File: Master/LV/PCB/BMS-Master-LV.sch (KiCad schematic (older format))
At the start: 24 parts, among them J10 Charge, J11 CAN, J12 USB, J13 Master, J18 OLED, J4 Power, J5 12V, J6 Power Button, J7 Cooling, J8 Discharge, K1 HE3621A1200, Q1 BSS138

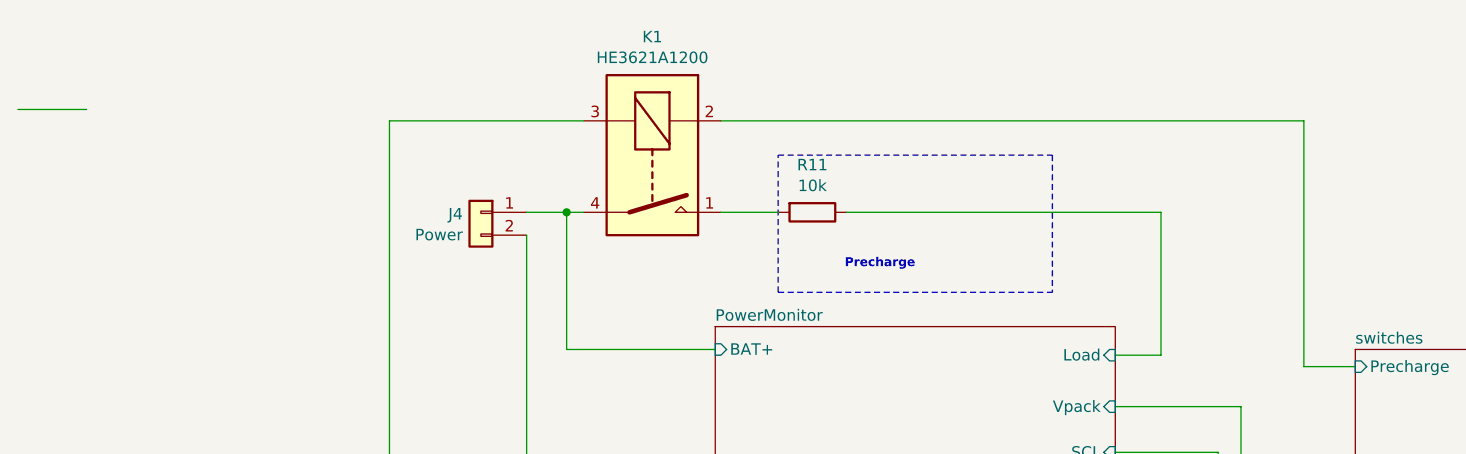
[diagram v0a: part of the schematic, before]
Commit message: maintenance update
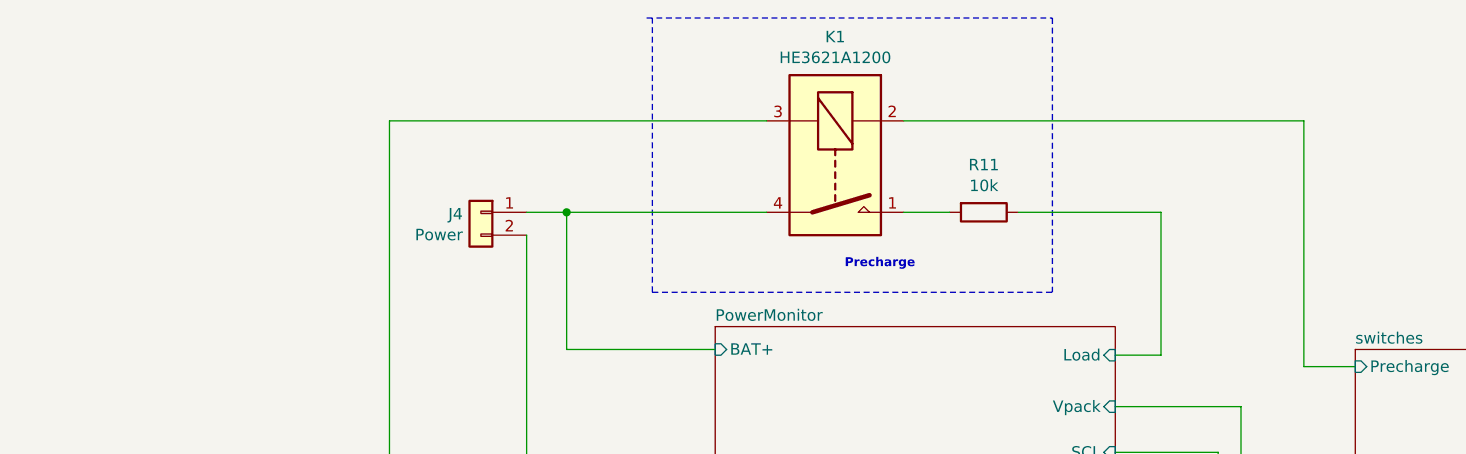
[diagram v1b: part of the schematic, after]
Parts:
- R11: MPN RC0603FR-0710KL -> 25121WJ0103T4E
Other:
- moved on the sheet: K1, R11
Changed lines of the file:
@@
 Precharge
 Wire Notes Line
-	4625 1350 4625 750
+	4075 1350 4075 150
 Wire Notes Line
-	4625 750  5825 750
+	4050 150  5825 150
 Wire Notes Line
-	5825 750  5825 1350
+	5825 150  5825 1350
 $Comp
 L power:+12V #PWR0112
@@
 ISOLATED
 Wire Notes Line
-	4625 1350 5825 1350
+	4075 1350 5825 1350
 Wire Wire Line
 	7100 5650 7150 5650
@@
 	-1   0    0    -1
 $EndComp
-Wire Wire Line
-	1300 550  1600 550
 $Sheet
 S 4350 1500 1750 1050
@@
 Connection ~ 3700 1000
 Wire Wire Line
-	3700 1000 3775 1000
-Wire Wire Line
 	2875 3600 2925 3600
 Wire Wire Line
@@
 Wire Wire Line
 	2925 3600 4125 3600
-Wire Wire Line
-	2925 600  3775 600
-$Comp
-L ENNOID:HE3621A1200 K1
-U 1 1 5DC5FBE0
-P 4075 800
-F 0 "K1" V 3508 800 50  0000 C CNN
-F 1 "HE3621A1200" V 3599 800 50  0000 C CNN
-F 2 "ENNOID:HE3621A1200" H 4425 750 50  0001 L CNN
-F 3 "" H 4075 800 50  0001 C CNN
-F 4 "HE3621A1200" H 4075 800 50  0001 C CNN "MPN"
-	1    4075 800
-	0    1    1    0
-$EndComp
-Wire Wire Line
-	4375 1000 4625 1000
-Wire Wire Line
-	4375 600  6925 600
 $Comp
 L Device:R R?
 U 1 1 5DC7CD7E
-P 4775 1000
+P 5525 1000
 AR Path="/5C519BA0/5DC7CD7E" Ref="R?"  Part="1"
 AR Path="/5D7DC460/5DC7CD7E" Ref="R?"  Part="1"
 AR Path="/5DC7CD7E" Ref="R11"  Part="1"
-F 0 "R11" V 4568 1000 50  0000 C CNN
-F 1 "10k" V 4659 1000 50  0000 C CNN
-F 2 "Resistor_SMD:R_2512_6332Metric" V 4705 1000 50  0001 C CNN
-F 3 "~" H 4775 1000 50  0001 C CNN
-F 4 "RC0603FR-0710KL" H 4775 1000 50  0001 C CNN "MPN"
-	1    4775 1000
+F 0 "R11" V 5318 1000 50  0000 C CNN
+F 1 "10k" V 5409 1000 50  0000 C CNN
+F 2 "Resistor_SMD:R_2512_6332Metric" V 5455 1000 50  0001 C CNN
+F 3 "~" H 5525 1000 50  0001 C CNN
+F 4 "25121WJ0103T4E" H 5525 1000 50  0001 C CNN "MPN"
+	1    5525 1000
 	0    1    1    0
 $EndComp
 Wire Wire Line
-	4925 1000 6300 1000
+	5675 1000 6300 1000
 $Sheet
 S 7150 3500 1550 6600
@@
 Wire Wire Line
 	4125 3600 4350 3600
+Wire Wire Line
+	3700 1000 4575 1000
+Wire Wire Line
+	5175 1000 5375 1000
+Wire Wire Line
+	5175 600  6925 600
+Wire Wire Line
+	2925 600  4575 600
+$Comp
+L ENNOID:HE3621A1200 K1
+U 1 1 5DC5FBE0
+P 4875 800
+F 0 "K1" V 4308 800 50  0000 C CNN
+F 1 "HE3621A1200" V 4399 800 50  0000 C CNN
+F 2 "ENNOID:HE3621A1200" H 5225 750 50  0001 L CNN
+F 3 "" H 4875 800 50  0001 C CNN
+F 4 "HE3621A1200" H 4875 800 50  0001 C CNN "MPN"
+	1    4875 800
+	0    1    1    0
+$EndComp
 $EndSCHEMATC
